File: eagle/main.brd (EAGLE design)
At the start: 49.2 x 49.5 mm, 34 parts, among them IC1 TS5205, Q1 SI4840DY, Q5 SI4840DY, U1 SN74AHC1G00DCKR, U2 SN74AHC1G00DCKR, U3 SN74AHC1G00DCKR

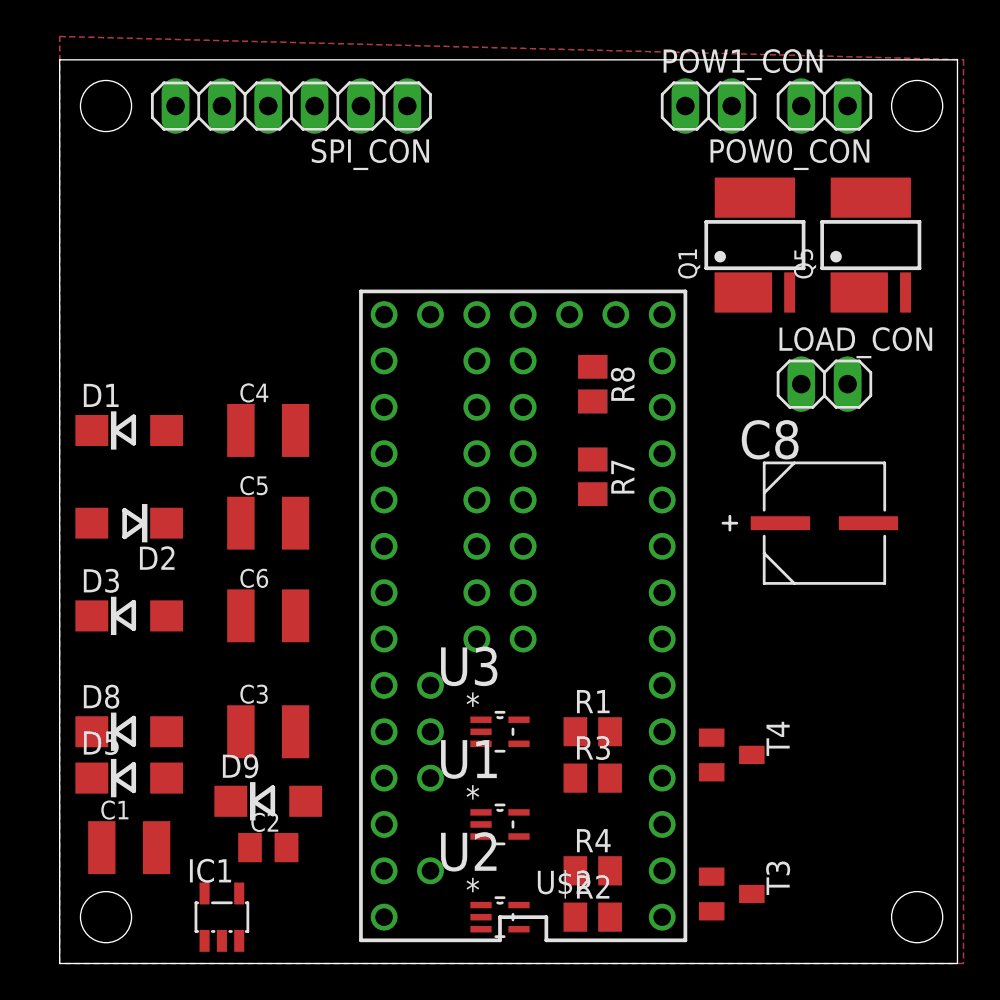
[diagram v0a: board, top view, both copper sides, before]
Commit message: routing
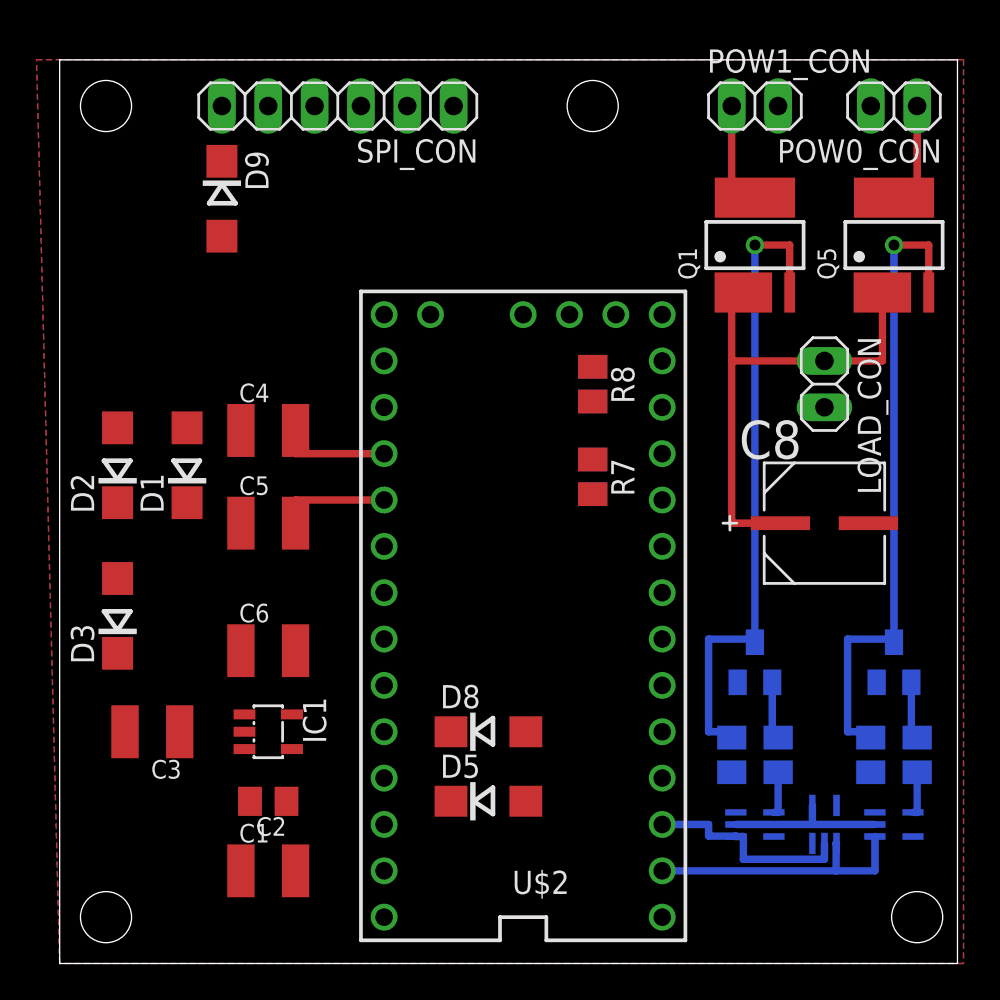
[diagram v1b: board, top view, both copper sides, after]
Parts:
- U$2: value TEENSY_3.0_ALLPINS -> TEENSY_3.0_BASIC-PGM; device Teensy3.0:TEENSY_3.0_ALLPINS -> Teensy3.0:TEENSY_3.0_BASIC-PGM
- moved D9 33.1 mm to (8.89, 41.9), turned to 270 degrees
- moved U2 22.2 mm to (45.7, 7.62), flipped to the bottom, turned to 180 degrees
- moved R2 19.9 mm to (47.0, 11.4), flipped to the bottom, turned to 90 degrees
- moved D5 19.7 mm to (23.5, 8.89)
- moved D8 19.7 mm to (23.5, 12.7)
- moved U1 17.8 mm to (41.9, 7.62), flipped to the bottom, turned to 90 degrees
- moved R4 16.5 mm to (44.5, 11.4), flipped to the bottom, turned to 90 degrees
- moved T3 15.5 mm to (45.7, 16.5), flipped to the bottom, turned to 0 degrees
- moved U3 14.9 mm to (38.1, 7.62), flipped to the bottom, turned to 180 degrees
- moved IC1 10.5 mm to (11.4, 12.7), turned to 270 degrees
- moved R1 10.2 mm to (39.4, 11.4), flipped to the bottom, turned to 90 degrees
- moved C1 7.73 mm to (11.4, 5.08)
- moved R3 7.73 mm to (36.8, 11.4), flipped to the bottom, turned to 90 degrees
- moved C3 6.35 mm to (5.08, 12.7), turned to 180 degrees
- moved T4 5.24 mm to (38.1, 16.5), flipped to the bottom, turned to 0 degrees
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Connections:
- removed net AREF: U$2.AREF
- removed net VUSB: U$2.VUSB
- net GND: no longer U$2.GND2
- net MCU_V+: no longer U$2.3.3V2
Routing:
- net N$1: track 0.00 -> 35.6 mm, vias 0 -> 1
- net N$2: track 0.00 -> 35.6 mm, vias 0 -> 1
- net LOAD_V+: track 0.00 -> 27.9 mm
- net POW0_EN: track 0.00 -> 15.1 mm
- net POW1_EN: track 0.00 -> 11.7 mm
- net XCOND_EN: track 0.00 -> 8.66 mm
- net POW1_V+: track 0.00 -> 6.41 mm
- net POW0_V+: track 0.00 -> 6.41 mm
- net PUMP_PWM#: track 0.00 -> 6.12 mm
- net PUMP_PWM: track 0.00 -> 6.12 mm
- net N$6: track 0.00 -> 3.35 mm
- net N$3: track 0.00 -> 3.35 mm
- net POW1_DIS: track 0.00 -> 2.43 mm
- net POW0_DIS: track 0.00 -> 2.43 mm
